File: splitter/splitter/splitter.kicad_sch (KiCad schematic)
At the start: 35 parts, among them J1 JACKIN, J10 Conn_01x08, J11 Conn_01x08, J2 JACKSEND, J3 JACKRECV, J4 JACKOUT, J5 Jack-DC, J6 JACKSEND2, J8 JACKRECV2, SW1 SW_MODE, SW2 SW_BYPASS, U1 TL074, U2 TLE2426xLP

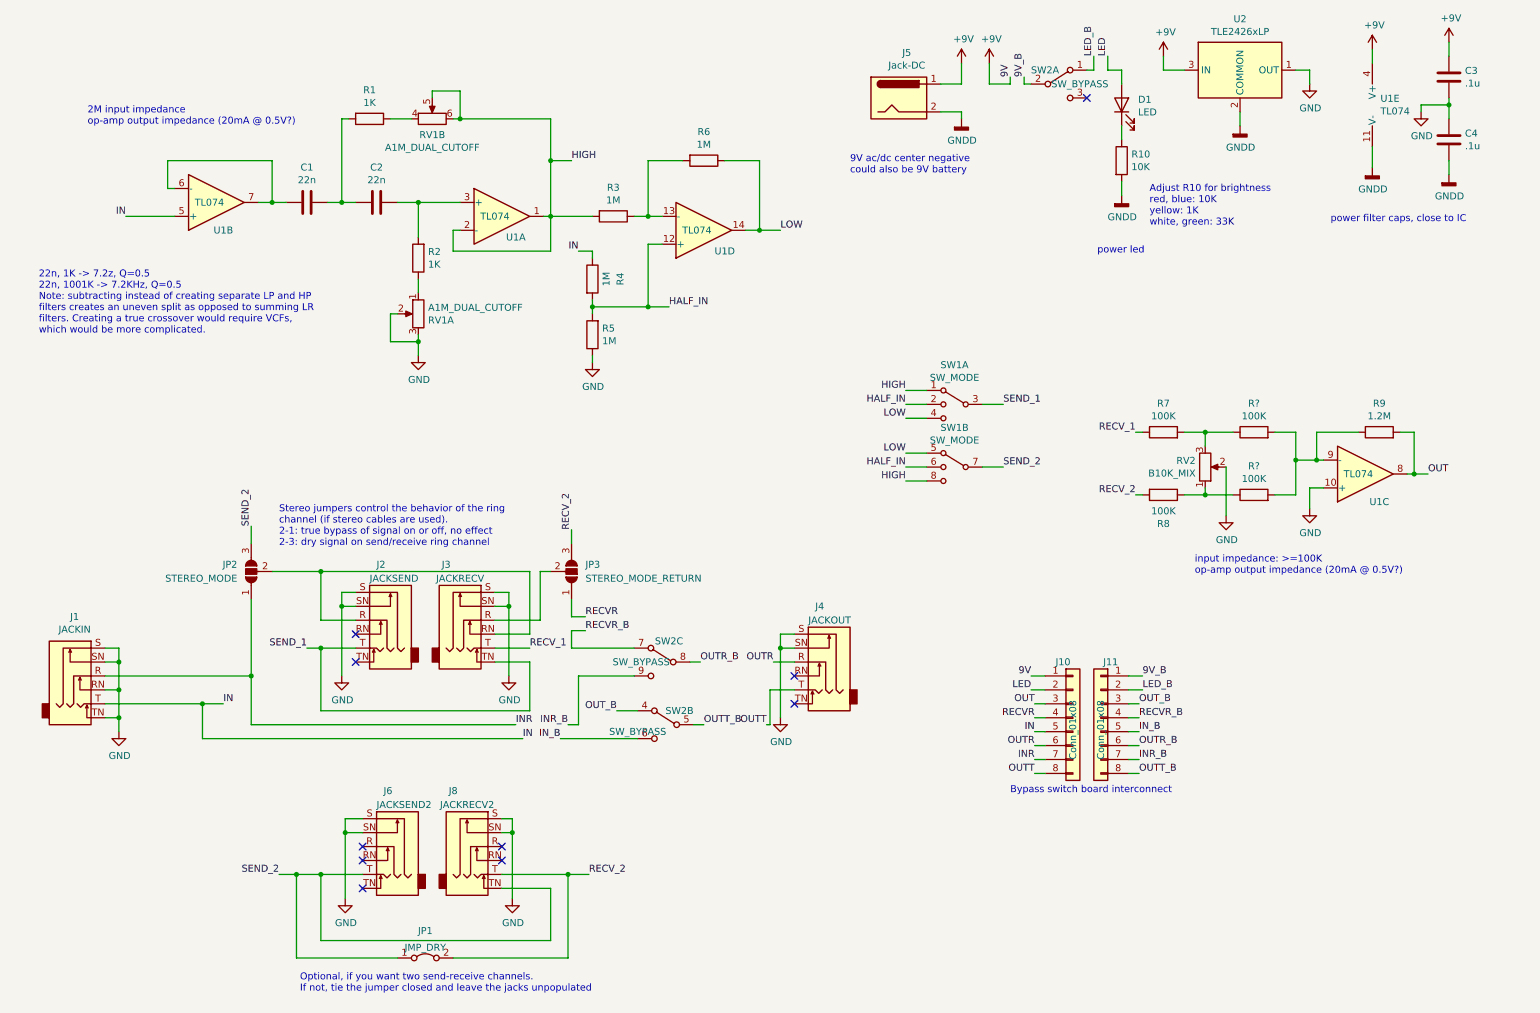
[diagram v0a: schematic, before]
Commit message: rev D
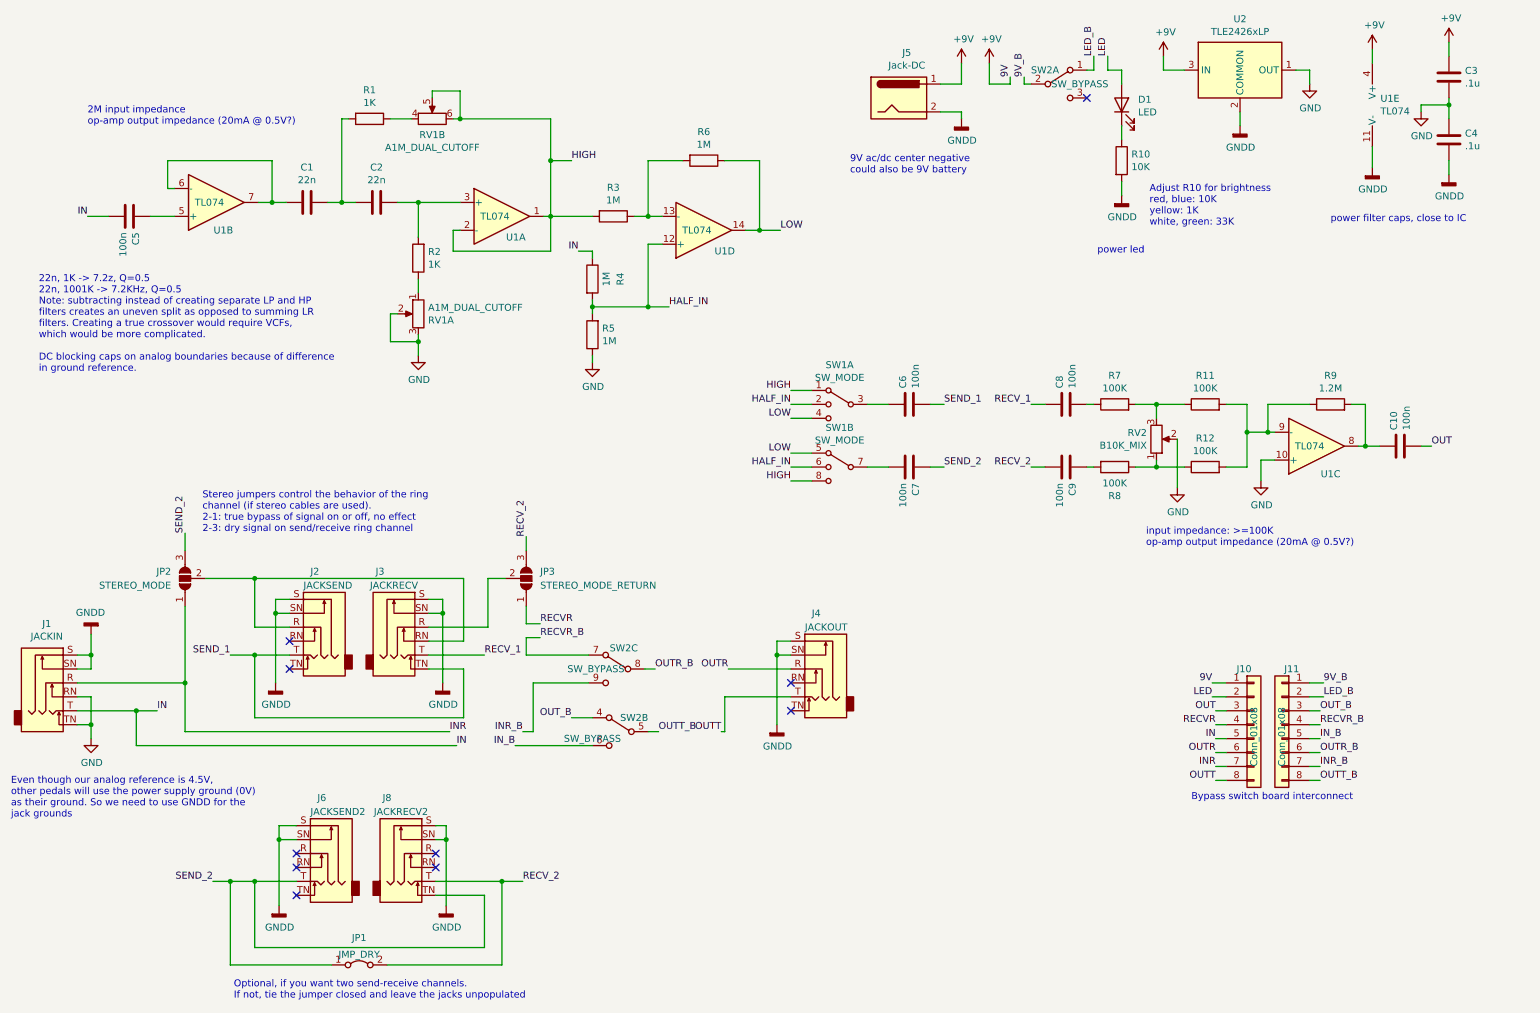
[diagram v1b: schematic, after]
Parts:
- added C10, C5, C6, C7, C8, C9: 100n, kicad-official/Capacitor_THT.pretty:C_Rect_L7.0mm_W2.5mm_P5.00mm, symbol Device:C
- C1, C2: footprint Capacitor_THT:C_Disc_D4.3mm_W1.9mm_P5.00mm -> kicad-official/Capacitor_THT.pretty:C_Disc_D4.3mm_W1.9mm_P5.00mm
- C3, C4: footprint Capacitor_THT:C_Rect_L7.0mm_W2.0mm_P5.00mm -> kicad-official/Capacitor_THT.pretty:CP_Radial_D5.0mm_P2.50mm
- D1: footprint LED_THT:LED_D3.0mm -> kicad-official/LED_THT.pretty:LED_D3.0mm
- J5: footprint Connector_PinSocket_2.54mm:PinSocket_1x02_P2.54mm_Vertical -> kicad-official/Connector_PinSocket_2.54mm.pretty:PinSocket_1x02_P2.54mm_Vertical
- JP1: footprint Jumper:SolderJumper-2_P1.3mm_Open_RoundedPad1.0x1.5mm -> kicad-official/Jumper.pretty:SolderJumper-2_P1.3mm_Open_RoundedPad1.0x1.5mm
- JP2, JP3: footprint (none) -> kicad-official/Jumper.pretty:SolderJumper-3_P1.3mm_Open_RoundedPad1.0x1.5mm
- R1, R10, R2, R3, R4, R5, R6, R7, R8, R9: footprint Resistor_THT:R_Axial_DIN0207_L6.3mm_D2.5mm_P7.62mm_Horizontal -> kicad-official/Resistor_THT.pretty:R_Axial_DIN0207_L6.3mm_D2.5mm_P7.62mm_Horizontal
- R11, R12: renamed from R?; footprint Resistor_THT:R_Axial_DIN0207_L6.3mm_D2.5mm_P7.62mm_Horizontal -> kicad-official/Resistor_THT.pretty:R_Axial_DIN0207_L6.3mm_D2.5mm_P7.62mm_Horizontal
- RV1: footprint Potentiometer_THT:Potentiometer_Alpha_RD902F-40-00D_Dual_Vertical -> kicad-official/Potentiometer_THT.pretty:Potentiometer_Alpha_RD902F-40-00D_Dual_Vertical
- RV2: footprint Potentiometer_THT:Potentiometer_Alpha_RD901F-40-00D_Single_Vertical -> kicad-official/Potentiometer_THT.pretty:Potentiometer_Alpha_RD901F-40-00D_Single_Vertical
- U1: footprint Package_DIP:DIP-14_W7.62mm -> kicad-official/Package_DIP.pretty:DIP-14_W7.62mm_Socket
- U2: footprint Package_TO_SOT_THT:TO-92_Inline_Wide -> kicad-official/Package_TO_SOT_THT.pretty:TO-92_Inline_Wide
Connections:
- net GND: no longer J1.S, J1.SN, J2.S, J2.SN, J3.S, J3.SN, J4.S, J4.SN, J6.S, J6.SN, J8.S, J8.SN
- net GNDD: now also J1.S, J1.SN, J2.S, J2.SN, J3.S, J3.SN, J4.S, J4.SN, J6.S, J6.SN, J8.S, J8.SN
- net IN: now also C5.2; no longer U1.5 (+)
- net OUT: now also C10.2; no longer R9.2, U1.8
- net RECV_1: now also C8.1; no longer R7.1
- net RECV_2: now also C9.2; no longer R8.2
- net SEND_1: now also C6.2; no longer SW1.3
- net SEND_2: now also C7.1; no longer SW1.7
- new net: C5.1, U1.5 (+)
- new net: C10.1, R9.2, U1.8
- new net: C9.1, R8.2
- new net: C8.2, R7.1
- new net: C6.1, SW1.3
- new net: C7.2, SW1.7
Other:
- note added: "22n, 1K -> 7.2z, Q=0.5 22n, 1001K -> 7.2KHz, Q=0.5 Note: subtracting instead of creating separate LP and HP filters creates an uneven split as opposed to summing LR filters. Creating a true crossover would require VCFs, which would be more complicated. DC blocking caps on analog boundaries because of difference in ground reference."
- note added: "Even though our analog reference is 4.5V, other pedals will use the power supply ground (0V) as their ground. So we need to use GNDD for the jack grounds"
- note removed: "22n, 1K -> 7.2z, Q=0.5 22n, 1001K -> 7.2KHz, Q=0.5 Note: subtracting instead of creating separate LP and HP filters creates an uneven split as opposed to summing LR filters. Creating a true crossover would require VCFs, which would be more complicated."
- moved on the sheet: J1, J10, J11, J2, J3, J4, J6, J8, JP1, JP2, JP3, R11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

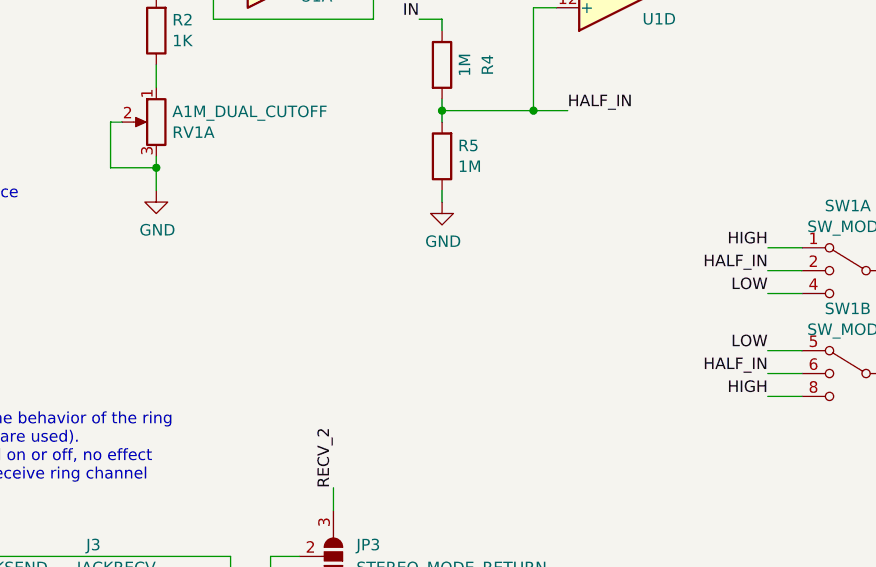
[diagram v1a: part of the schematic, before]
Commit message: mechanicals and measurements
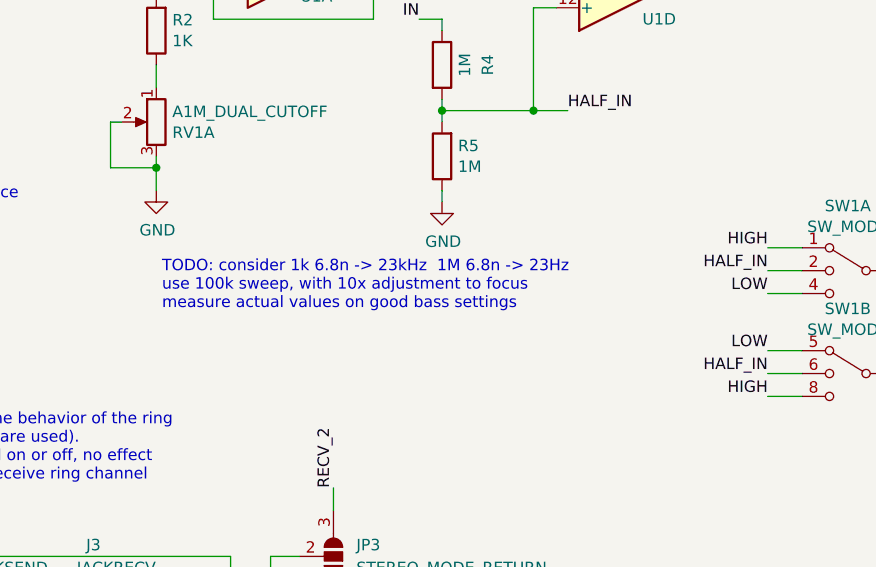
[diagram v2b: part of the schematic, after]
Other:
- note added: "TODO: consider 1k 6.8n -> 23kHz 1M 6.8n -> 23Hz use 100k sweep, with 10x adjustment to focus measure actual values on good bass settings"
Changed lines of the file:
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@@
+    (effects (font (size 1.27 1.27)) (justify left bottom))
+  )
+  (text "TODO: consider 1k 6.8n -> 23kHz  1M 6.8n -> 23Hz\nuse 100k sweep, with 10x adjustment to focus\nmeasure actual values on good bass settings"
+    (at 89.535 89.535 0)
     (effects (font (size 1.27 1.27)) (justify left bottom))
   )
